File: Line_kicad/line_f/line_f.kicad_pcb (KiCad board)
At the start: 2 copper layers, 135 x 157.5 mm, 16 parts, among them M2 Motor_DC, M3 Motor_DC, SW1 SW_SPST, SW2 SW_SPDT, SW3 SW_Push, SW4 SW_Push, U1 TB6612FNG_LINE, m1 BLACKPILL

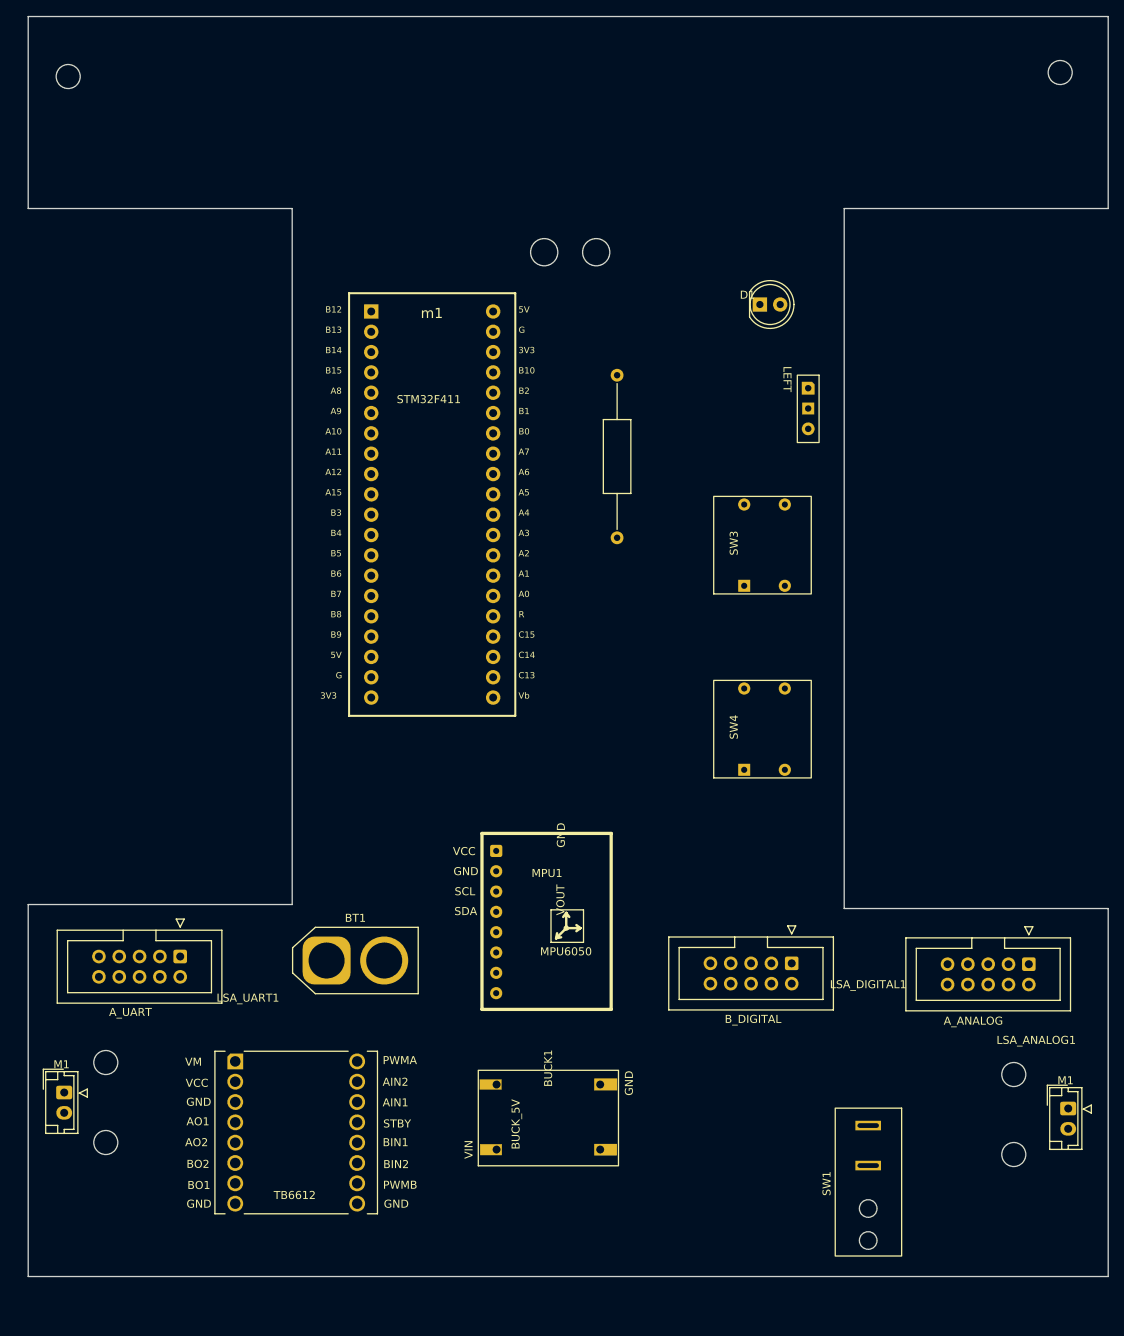
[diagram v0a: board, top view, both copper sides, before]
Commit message: 3#
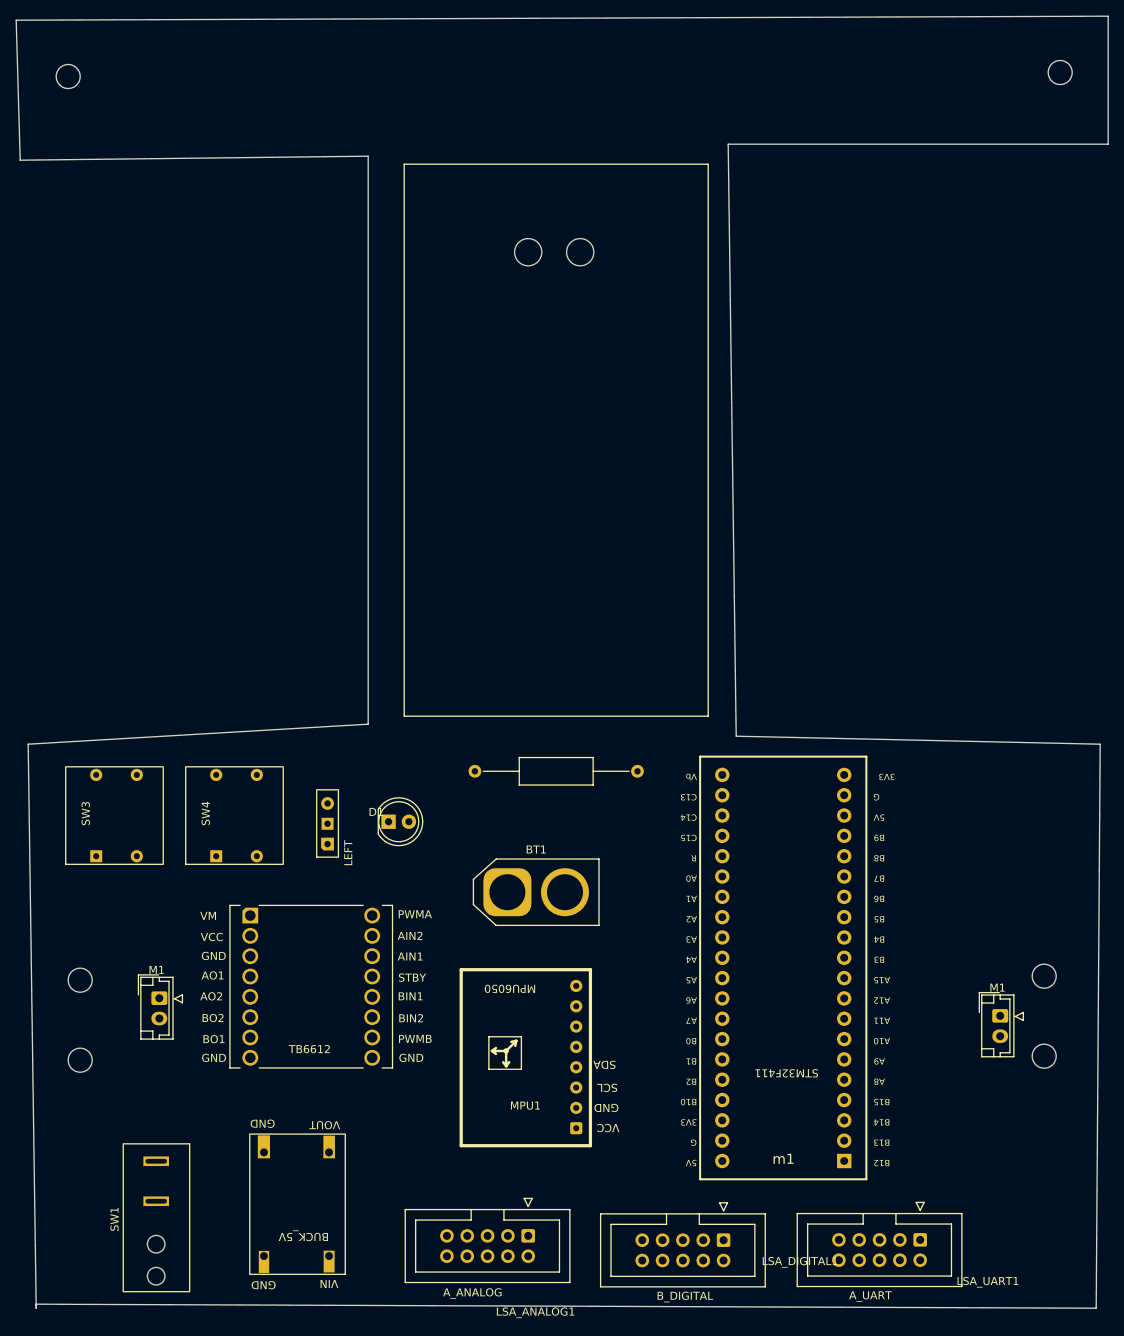
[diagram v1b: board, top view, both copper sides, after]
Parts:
- moved LSA_UART1 99.0 mm to (144.2, 185.6)
- moved SW1 89.1 mm to (41.5, 176.8)
- moved SW3 87.8 mm to (36.0, 126.9)
- moved D1 79.6 mm to (72.0, 132.0)
- moved SW2 74.9 mm to (66.0, 127.5), turned to 90 degrees
- moved m1 72.7 mm to (119.9, 145.5), turned to 180 degrees
- moved LSA_ANALOG1 71.2 mm to (96.7, 178.2)
- moved SW4 66.9 mm to (51.0, 126.9)
- moved BUCK1 52.4 mm to (45.8, 171.4), turned to 180 degrees
- moved R1 43.2 mm to (91.7, 124.7), turned to 0 degrees
- moved LSA_DIGITAL1 35.6 mm to (122.0, 182.7)
- moved BT1 24.2 mm to (85.4, 136.0)
- moved U1 18.3 mm to (60.9, 147.8)
- moved M2 16.7 mm to (37.4, 150.6)
- moved MPU1 14.4 mm to (95.8, 145.7), turned to 180 degrees
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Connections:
- M2 pad 1: AO1 -> (no net)
- M2 pad 2: AO2 -> (no net)
- M3 pad 1: BO1 -> (no net)
- M3 pad 2: BO2 -> (no net)
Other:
- board size 135 x 157.5 mm -> 136.5 x 161.5 mm
